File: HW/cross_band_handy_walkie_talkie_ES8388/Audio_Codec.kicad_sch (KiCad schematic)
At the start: 46 parts

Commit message: t
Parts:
- removed C? (x6): 1u, Capacitor_SMD:C_0603_1608Metric_Pad1.08x0.95mm_HandSolder, symbol Device:C_Small
- removed C? (x6): 100n, Capacitor_SMD:C_0603_1608Metric_Pad1.08x0.95mm_HandSolder, symbol Device:C_Small
- removed C? (x3): 10u, Capacitor_SMD:C_0805_2012Metric, symbol Device:C_Small
- removed J? (x2): AUDIO, Connector_PinHeader_2.54mm:PinHeader_1x03_P2.54mm_Vertical, symbol Connector_Generic:Conn_01x03
- removed R? (x7): 1k, Resistor_SMD:R_0603_1608Metric_Pad0.98x0.95mm_HandSolder, symbol Device:R_Small
- removed R?: 2k7, Resistor_SMD:R_0603_1608Metric_Pad0.98x0.95mm_HandSolder, symbol Device:R_Small
- removed TP?: TestPoint_THT, TestPoint:TestPoint_Loop_D2.60mm_Drill0.9mm_Beaded, symbol Connector:TestPoint
- removed U?: TLV320AIC3254, Package_DFN_QFN:QFN-32-1EP_5x5mm_P0.5mm_EP3.1x3.1mm_ThermalVias, symbol My_custom_lib:TLV320AIC3254
- added C24, C25, C27, C28, C30, C31, C34, C35, C? (x6): 1u, Capacitor_SMD:C_0603_1608Metric_Pad1.08x0.95mm_HandSolder, symbol Device:C_Small
- added C? (x8): 10u, Capacitor_SMD:C_0805_2012Metric, symbol Device:C_Small
- added JP1: 3p, Jumper:SolderJumper-3_P1.3mm_Bridged12_Pad1.0x1.5mm, symbol Jumper:Jumper_3_Bridged12
- gave numbers to parts that had none: 19
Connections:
- net +3V3: now also U6.2 (DVDD), U6.3 (PVDD), C?.1, C?.1, C?.2, C?.2, JP1.3 (B); no longer C32.1, C33.1
- net +5V: now also C?.1, C?.1
- net BCLK: now also U6.5 (SCLK)
- net DIN: now also U6.6 (DSDIN)
- net DOUT: now also U6.8 (ASDOUT)
- net GND: now also U6.13 (HPGND), C?.1, C?.1, C?.1, C?.1, C?.1, C?.1, C?.2, C?.2, C?.2, C?.2, C?.2, C?.2, C?.2, C?.2, JP1.1 (A); no longer U6.17 (AVDD)
- net MCLK: now also U6.1 (MCLK)
- net SCL: now also U6.28 (CCLK)
- net SDA: now also U6.27 (CDATA)
- net WCLK: now also U6.7 (LRCK)
- net at C29.1, J5.T: no longer R28.1
- net at R31.1: no longer R30.1
- net at L1.2, U5.9 (AVDD): now also C?.1
- net at U6.10 (VREF): now also C?.1
- net at U6.11 (ROUT1): now also C31.2
- net at U6.12 (LOUT1): now also C30.2
- net at U6.14 (ROUT2): now also C34.1
- net at U6.15 (LOUT2): now also C35.1
- net at U6.16 (HPVDD): now also C?.1, C?.2
- net at U6.19 (ADCVREF): now also C32.1, C?.2
- net at U6.20 (VMID): now also C33.1, C?.2
- net at U6.21 (RIN2): now also C28.1
- net at U6.22 (LIN2): now also C27.1
- net at U6.23 (RIN1): now also C25.1
- net at U6.24 (LIN1): now also C24.1
- net at U6.26 (CE): now also JP1.2 (C)
- new net: C?.1, C?.2, U6.17 (AVDD)
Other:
- note removed: "0011000"
- moved on the sheet: C16, C18, C19, C20, C21, C22, C23, C26, C29, C32, C33, J5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

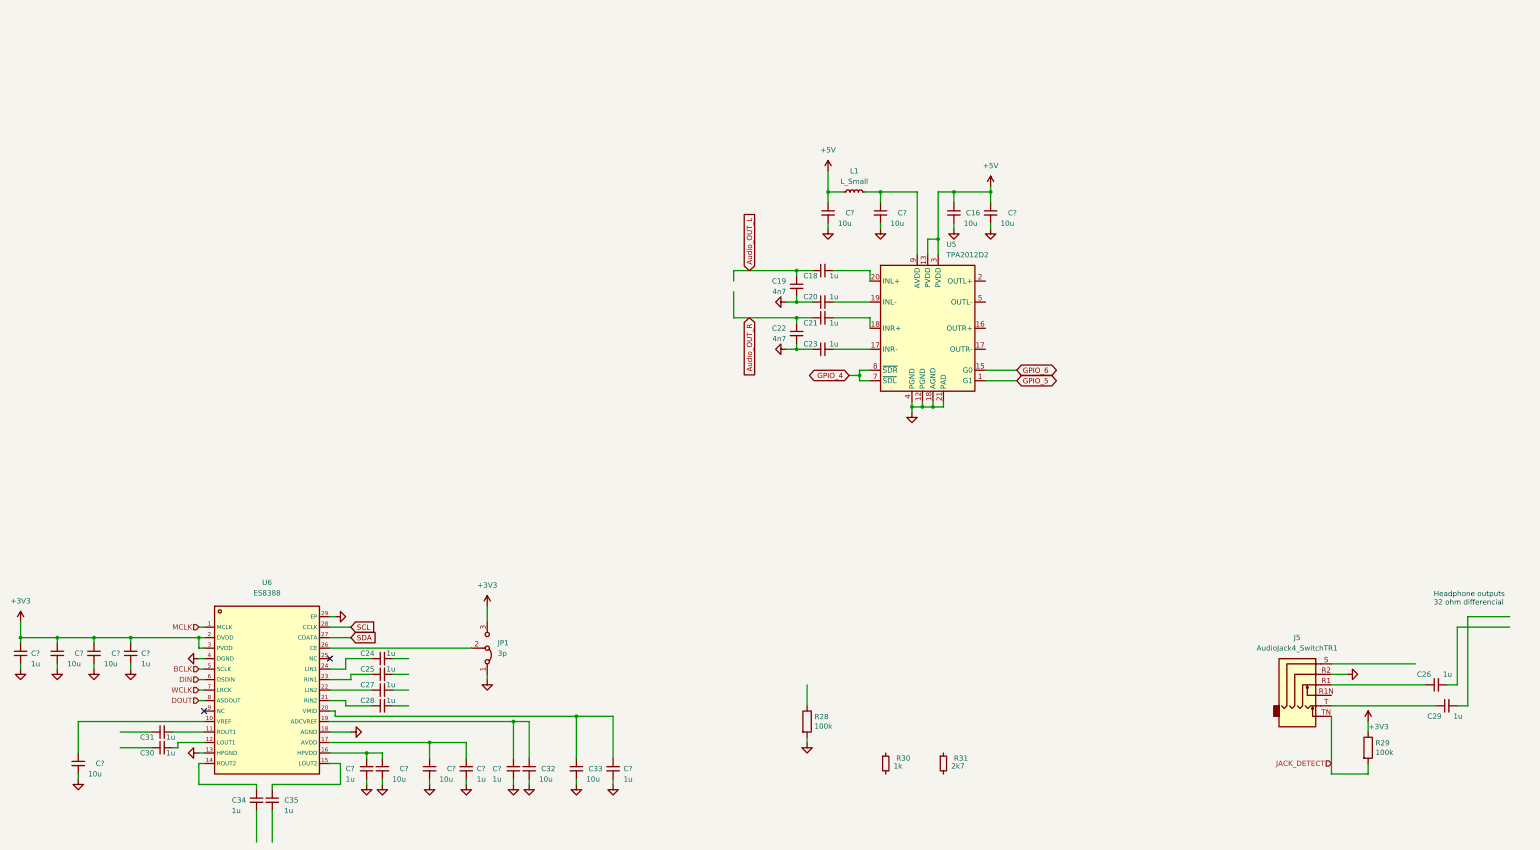
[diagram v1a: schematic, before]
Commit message: b
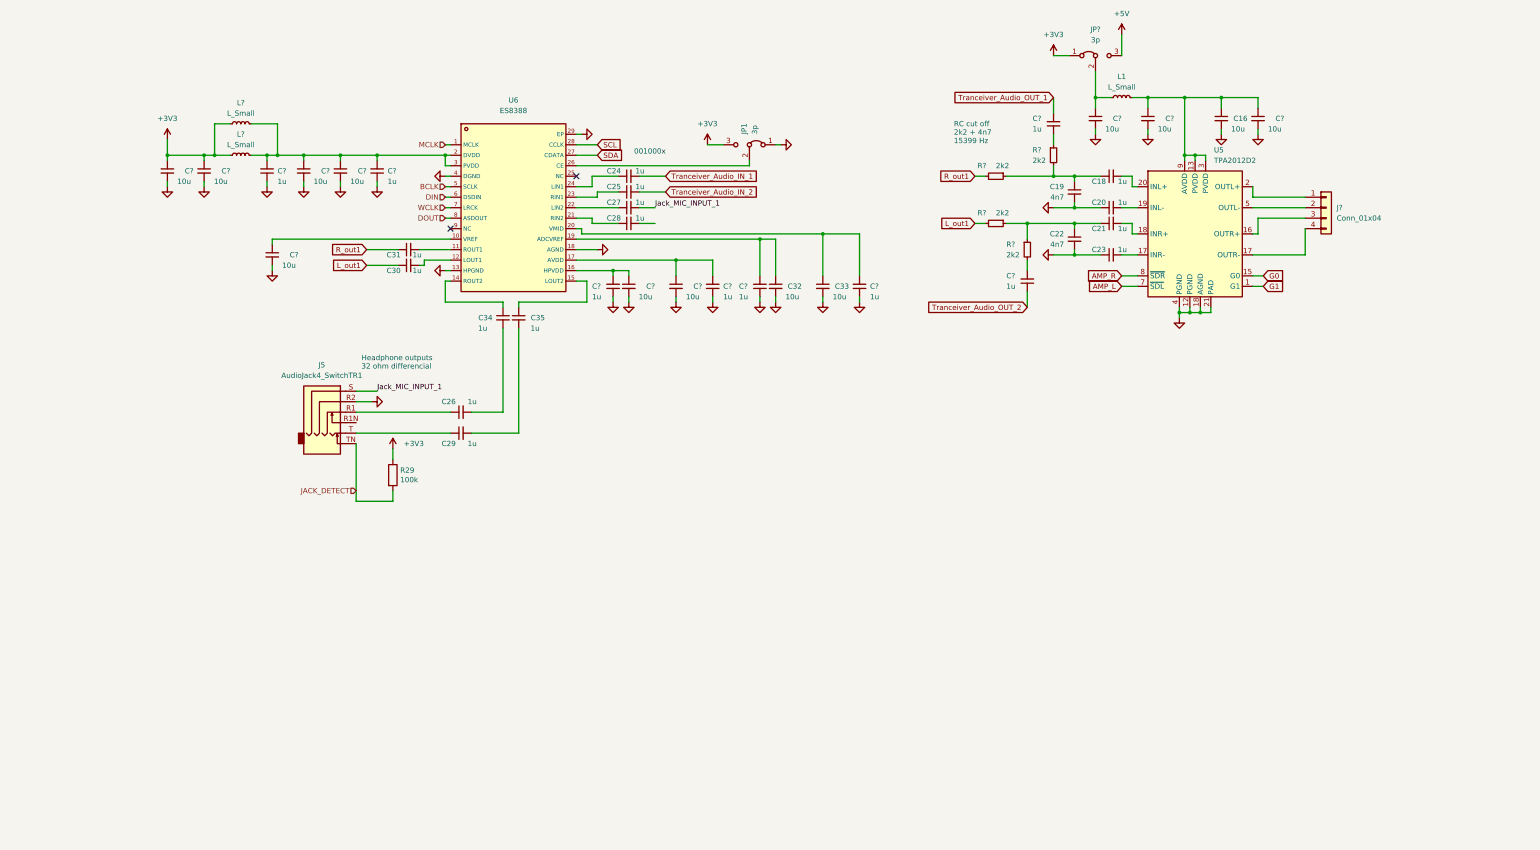
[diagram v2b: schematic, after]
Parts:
- removed R28: 100k, Resistor_SMD:R_0805_2012Metric, symbol Device:R
- removed R30: 1k, Resistor_SMD:R_0603_1608Metric_Pad0.98x0.95mm_HandSolder, symbol Device:R_Small
- removed R31: 2k7, Resistor_SMD:R_0603_1608Metric_Pad0.98x0.95mm_HandSolder, symbol Device:R_Small
- added C? (x2): 10u, Capacitor_SMD:C_0805_2012Metric, symbol Device:C_Small
- added C? (x2): 1u, Capacitor_SMD:C_0603_1608Metric_Pad1.08x0.95mm_HandSolder, symbol Device:C_Small
- added J?: Conn_01x04, symbol Connector_Generic:Conn_01x04
- added JP?: 3p, Jumper:SolderJumper-3_P1.3mm_Bridged12_Pad1.0x1.5mm, symbol Jumper:Jumper_3_Bridged12
- added L? (x2): L_Small, Inductor_SMD:L_0603_1608Metric, symbol Device:L_Small
- added R? (x4): 2k2, Resistor_SMD:R_0603_1608Metric_Pad0.98x0.95mm_HandSolder, symbol Device:R_Small
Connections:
- net +3V3: now also C?.1, C?.1, JP?.1 (A), L?.1, L?.1; no longer C?.1, C?.1, C?.2, C?.2, U6.2 (DVDD), U6.3 (PVDD)
- net +5V: now also JP?.3 (B); no longer C16.1, C?.1, C?.1, L1.1, U5.13 (PVDD), U5.3 (PVDD)
- net GND: now also C?.2, C?.2
- net L_out1: now reaches C30.1
- net L_out1: now also R?.2
- net Jack_MIC_INPUT_1: now reaches J5.S
- net Jack_MIC_INPUT_1: now also C27.2
- net at C34.2: now also C26.2
- net at U5.16 (OUTR+): now also J?.3 (Pin_3)
- net at U5.17 (OUTR-): now also J?.4 (Pin_4)
- net at U5.2 (OUTL+): now also J?.1 (Pin_1)
- net at U5.5 (OUTL-): now also J?.2 (Pin_2)
- net at C?.1, L1.2, U5.9 (AVDD): now also C16.1, C?.1, U5.13 (PVDD), U5.3 (PVDD)
- net at C29.2: now also C35.2
- net R_out1: now reaches C31.1
- net R_out1: now also R?.2
- net Tranceiver_Audio_IN_2: now reaches C25.2
- net Tranceiver_Audio_IN_1: now reaches C24.2
- net Audio_OUT_L: no longer names the net of C18.1, C19.1
- net Audio_OUT_L: now also R?.1, R?.2
- net Audio_OUT_R: no longer names the net of C21.1, C22.1
- net Audio_OUT_R: now also R?.1, R?.1
- net GPIO_4 renamed AMP_L
- net AMP_L: no longer U5.8 (~{SDR})
- net GPIO_5 renamed G1
- net GPIO_6 renamed G0
- new net: C?.1, C?.1, C?.2, C?.2, L?.2, L?.2, U6.2 (DVDD), U6.3 (PVDD)
- new net: C?.1, R?.1
- new net: C?.1, JP?.2 (C), L1.1
- new net: C?.2, R?.2
- new net AMP_R: U5.8 (~{SDR})
- new net Tranceiver_Audio_OUT_1: C?.2
- new net Tranceiver_Audio_OUT_2: C?.1
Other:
- note added: "001000x"
- note added: "RC cut off 2k2 + 4n7 15399 Hz"
- moved on the sheet: C16, C18, C19, C20, C21, C22, C23, C24, C25, C26, C27, C28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
